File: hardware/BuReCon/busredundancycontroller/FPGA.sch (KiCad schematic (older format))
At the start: 19 parts, among them U1 ICE40LP1K-CM36, U8 SST26VF032B

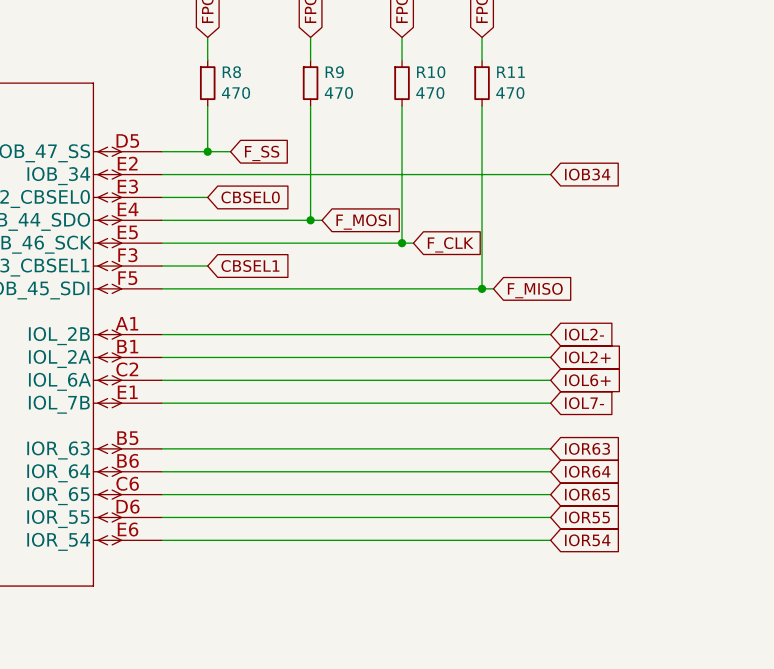
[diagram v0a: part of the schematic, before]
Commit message: Connectors and RS232
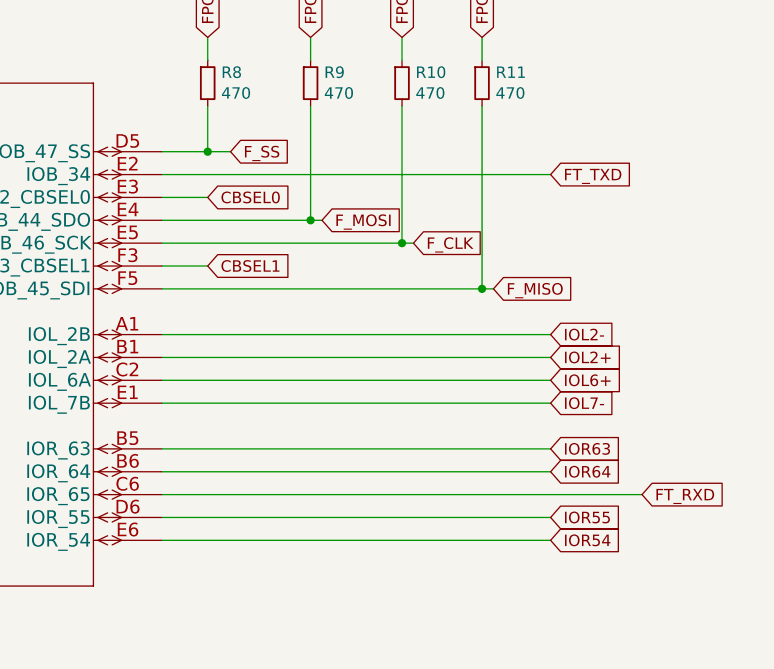
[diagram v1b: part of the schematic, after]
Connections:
- net IOB34 renamed FT_TXD
- net IOR65 renamed FT_RXD
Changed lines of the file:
@@
 Text GLabel 3850 3800 0    50   Input ~ 0
 GCLOCK
-Text GLabel 9250 2500 2    50   Input ~ 0
-IOB34
 Wire Wire Line
 	7550 2500 9250 2500
@@
 Text GLabel 9250 3800 2    50   Input ~ 0
 IOR64
-Text GLabel 9250 3900 2    50   Input ~ 0
-IOR65
 Text GLabel 9250 4000 2    50   Input ~ 0
 IOR55
@@
 Wire Wire Line
 	7550 3800 9250 3800
-Wire Wire Line
-	7550 3900 9250 3900
 Wire Wire Line
 	7550 4000 9250 4000
@@
 Wire Wire Line
 	4150 3900 4550 3900
+Text GLabel 9650 3900 2    50   Input ~ 0
+FT_RXD
+Wire Wire Line
+	7550 3900 9650 3900
+Text GLabel 9250 2500 2    50   Input ~ 0
+FT_TXD
 $EndSCHEMATC
